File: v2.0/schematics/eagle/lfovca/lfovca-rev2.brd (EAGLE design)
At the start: 98.7 x 54.6 mm, 66 parts, among them IC1 TL082P, IC2 TL084P, T1 2N3904, T2 2N3904, T3 2N3904, T4 BC547, T5 BC547, T6 BC547

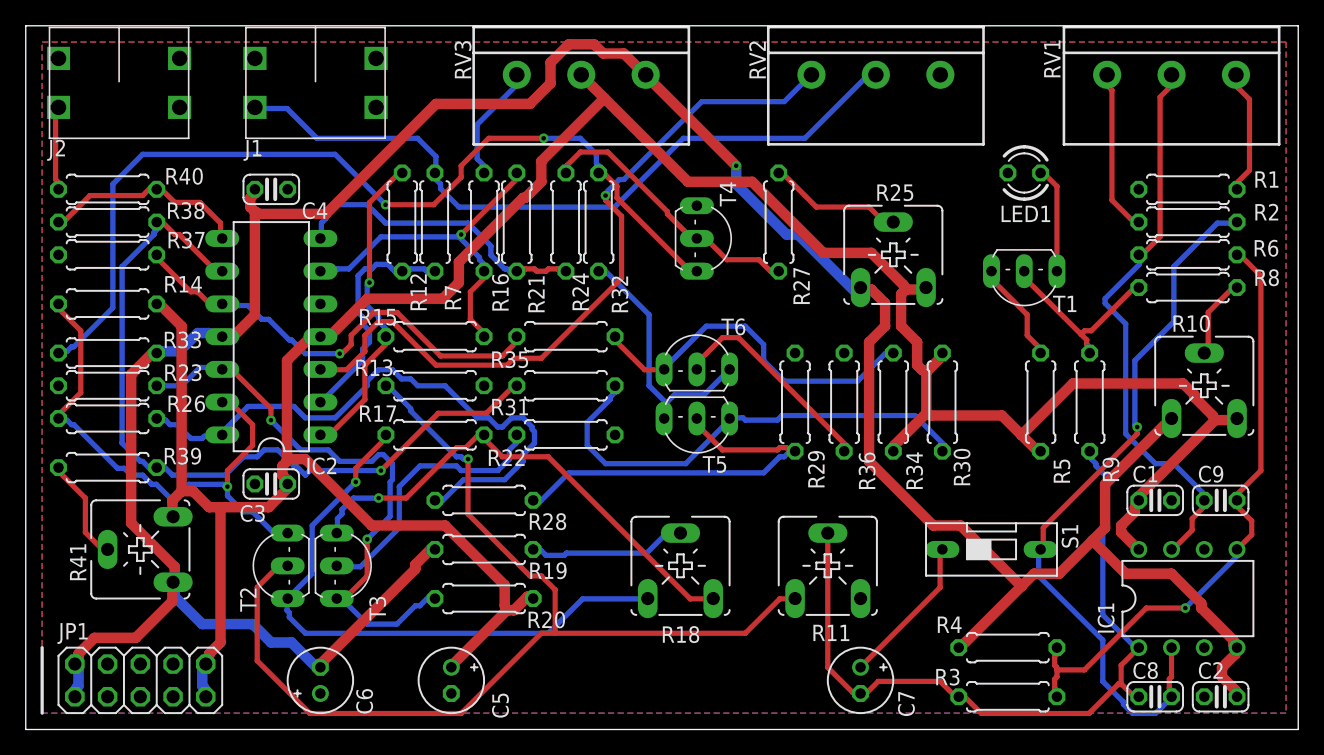
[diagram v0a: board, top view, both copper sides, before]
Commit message: LFOVCA: Optimize routes; cam outputs
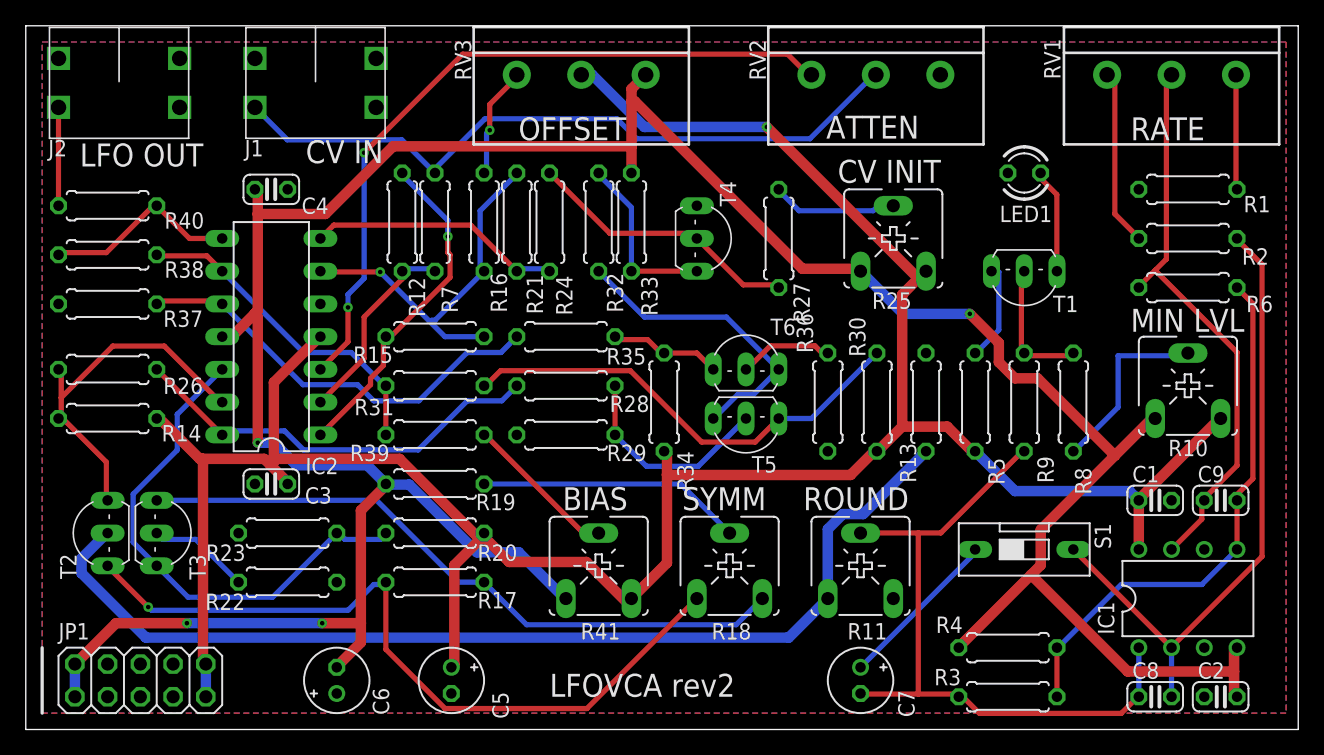
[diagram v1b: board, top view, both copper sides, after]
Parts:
- moved R33 41.9 mm to (47.0, 39.4), turned to 270 degrees
- moved R13 38.1 mm to (69.8, 25.4), turned to 270 degrees
- moved R41 35.6 mm to (44.5, 12.7), turned to 0 degrees
- moved R39 25.5 mm to (31.8, 22.9), turned to 0 degrees
- moved R22 24.4 mm to (20.3, 11.4)
- moved R23 18.1 mm to (20.3, 15.2)
- moved R29 18.0 mm to (41.9, 22.9), turned to 0 degrees
- moved R34 17.8 mm to (49.5, 25.4)
- moved T2 14.2 mm to (5.08, 15.2)
- moved T3 14.2 mm to (11.4, 15.2)
- moved R8 12.6 mm to (81.3, 25.4), turned to 270 degrees
- moved R17 11.4 mm to (31.8, 11.4)
- moved R28 10.9 mm to (41.9, 26.7)
- moved R31 10.2 mm to (31.8, 26.7)
- moved R14 8.89 mm to (6.35, 24.1)
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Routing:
- net N$15: track 71.4 -> 13.8 mm, vias 2 -> 0
- net N$7: track 61.2 -> 25.8 mm, vias 1 -> 0
- net N$11: track 27.7 -> 9.05 mm
- net +12V: track 213.3 -> 198.5 mm, vias 0 -> 1
- net N$19: track 31.0 -> 16.5 mm
- net N$28: track 42.0 -> 27.9 mm, vias 1 -> 0
- net N$26: track 46.8 -> 32.8 mm
- net N$29: track 21.2 -> 7.93 mm
- net N$31: track 38.7 -> 51.8 mm, vias 1 -> 0
- net N$30: track 47.0 -> 58.7 mm
- net N$25: track 16.9 -> 7.34 mm
- net -12V: track 221.2 -> 230.2 mm, vias 1 -> 4
- net N$33: track 12.3 -> 20.6 mm
- net N$34: track 6.33 -> 14.4 mm
- net N$8: track 56.1 -> 50.0 mm, vias 1 -> 0
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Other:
- board text added: "ATTEN"
- board text added: "BIAS"
- board text added: "CV IN"
- board text added: "CV INIT"
- board text added: "LFO OUT"
- board text added: "LFOVCA rev2"
- board text added: "MIN LVL"
- board text added: "OFFSET"
- board text added: "RATE"
- board text added: "ROUND"
- board text added: "SYMM"
